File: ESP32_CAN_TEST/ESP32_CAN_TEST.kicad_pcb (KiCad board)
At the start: 2 copper layers, 45.8 x 45.8 mm, 35 parts, among them J1 XT60, J2 Encoder_1, J3 Molex_2x2, J4 Encoder2, J5 Molex_2x2, J6 UART, J7 GH1.25, SW1 EN, SW2 EN, U1 AMS1117, U2 ESP32-WROOM-32, U3 MP1584, U4 TJA1051T, U5 TJA1051T

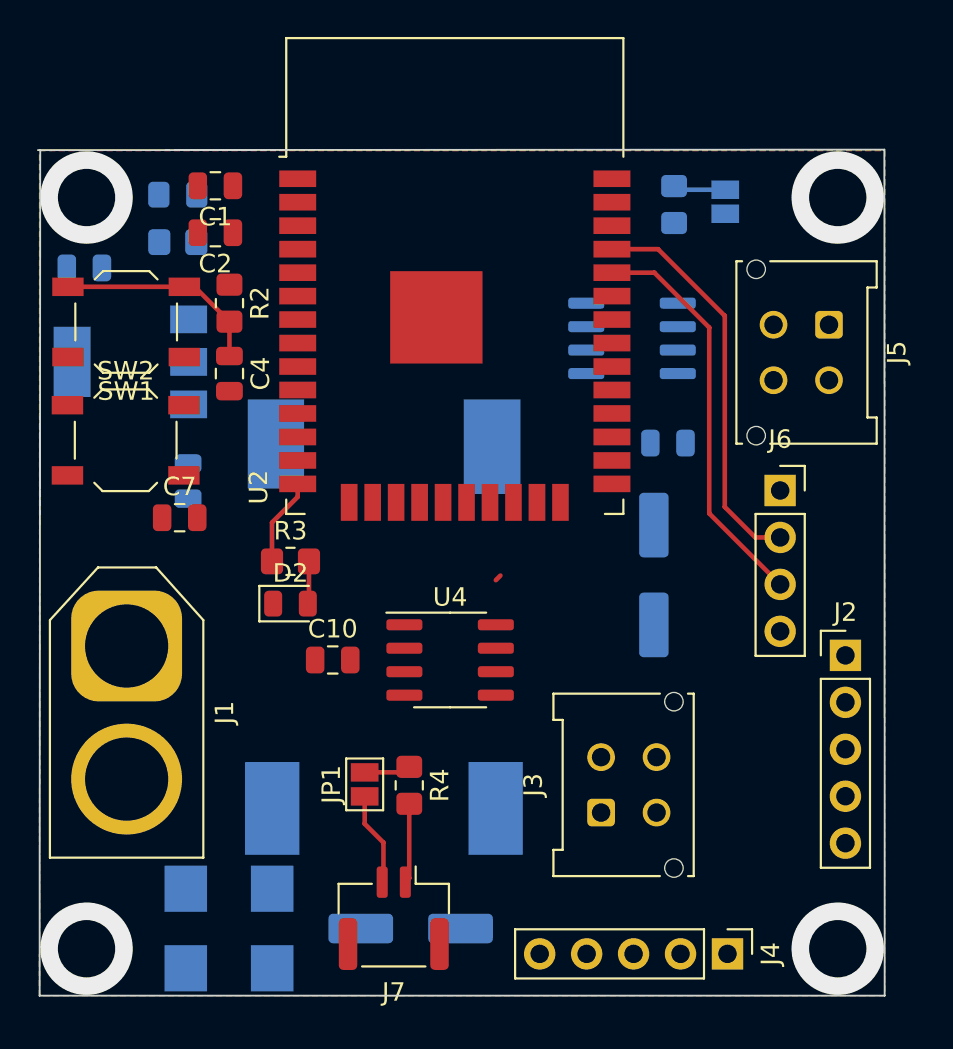
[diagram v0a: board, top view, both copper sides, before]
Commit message: new esp
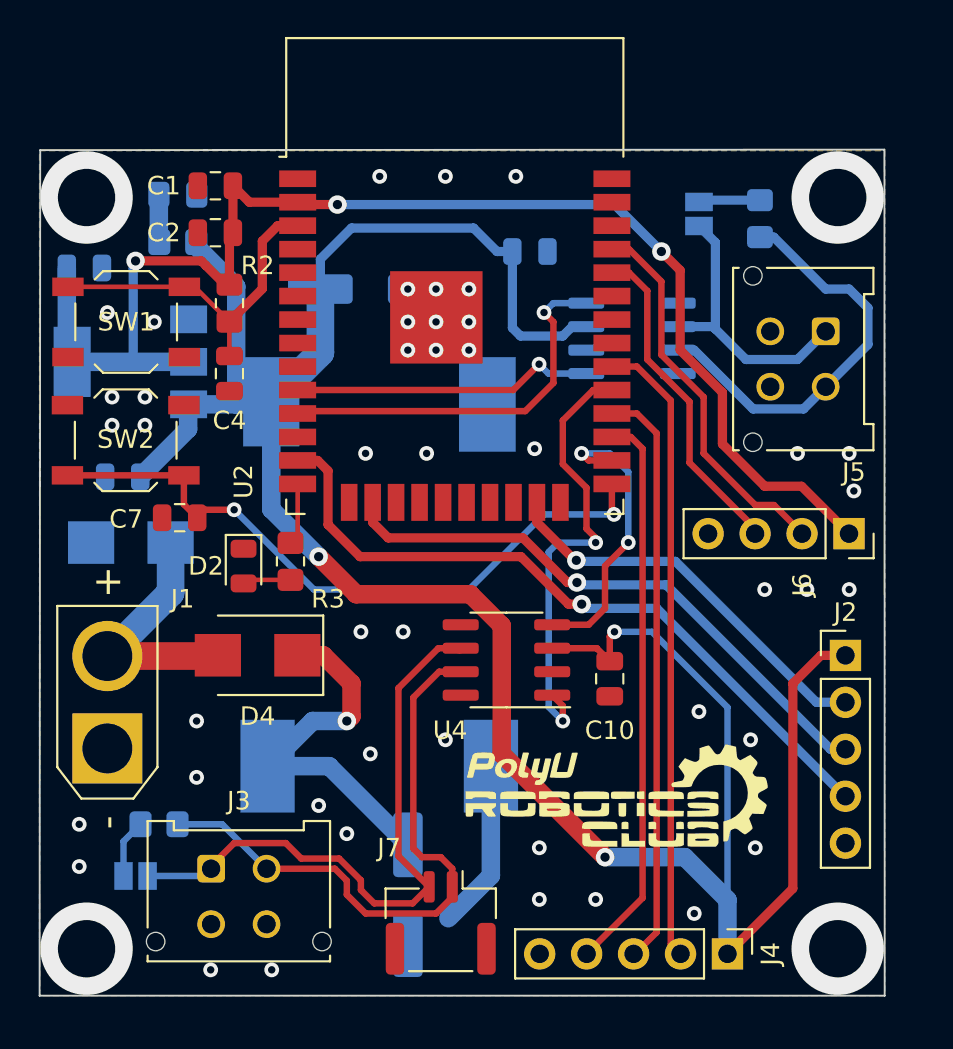
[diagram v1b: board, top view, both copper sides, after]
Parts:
- added G***: LOGO, PolyuRobotics:Club_logo, F.Cu at (138.2, 111.5)
- D4: moved to F.Cu
- J1: footprint Connector_AMASS:AMASS_XT60-M_1x02_P7.20mm_Vertical -> Connector_AMASS:AMASS_XT30U-M_1x02_P5.0mm_Vertical
- JP1, R4: moved to B.Cu
- moved C9 21.8 mm to (124.7, 83.8), turned to 0 degrees
- moved J3 21.3 mm to (116.1, 115.2), turned to 0 degrees
- moved D3 21.1 mm to (111.8, 97.5), turned to 0 degrees
- moved C10 15.0 mm to (137.7, 104.9), turned to 90 degrees
- moved D4 14.8 mm to (118.6, 103.6), turned to 180 degrees
- moved R4 13.7 mm to (113.3, 112.8), turned to 0 degrees
- moved JP1 13.3 mm to (112.0, 115.6), turned to 180 degrees
- moved C12 12.8 mm to (133.3, 81.8)
- moved J1 5.64 mm to (110.5, 108.7), turned to 90 degrees
- moved R9 4.71 mm to (145.8, 80.0)
- moved J6 4.40 mm to (150.6, 97.1), turned to -90 degrees
- moved C3 3.55 mm to (111.3, 94.0), turned to 180 degrees
- moved D2 3.25 mm to (117.9, 98.8), turned to -90 degrees
- moved U4 3.05 mm to (132.1, 103.9), turned to 180 degrees
- moved J7 2.55 mm to (128.5, 118.1)
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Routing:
- net +5V: track 0.00 -> 140.2 mm, vias 0 -> 3
- net +3V3: track 0.00 -> 73.3 mm, vias 0 -> 3
- net /IO14: track 0.00 -> 38.9 mm, vias 0 -> 1
- net Net-(C7-Pad2): track 0.35 -> 36.8 mm, vias 0 -> 2
- net /IO18: track 0.00 -> 34.1 mm
- net /IO17: track 0.00 -> 31.9 mm
- net /IO13: track 0.00 -> 31.7 mm, vias 0 -> 1
- net /IO16: track 0.00 -> 30.5 mm
- net /CANH+: track 5.09 -> 33.9 mm
- net /CANL-: track 4.33 -> 33.1 mm
- net /CAN_TX: track 0.00 -> 24.5 mm, vias 0 -> 2
- net /CAN2L-: track 0.00 -> 23.1 mm
- net /IO15: track 0.00 -> 21.8 mm, vias 0 -> 1
- net /CAN2_RX: track 0.00 -> 21.0 mm, vias 0 -> 1
- net Net-(C6-Pad1): track 0.00 -> 20.4 mm, vias 0 -> 1
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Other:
- board size 45.8 x 45.8 mm -> 45.7 x 45.8 mm
- board text added: "ESP32 Test Board Samson Chau Rev 2.0 2022-6-23"
